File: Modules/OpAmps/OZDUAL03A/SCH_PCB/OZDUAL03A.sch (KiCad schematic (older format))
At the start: 53 parts, among them J1 JUMP2_2x1, J2 POWER, J3 OPAMPA, J4 OPAMPB, J5 VREF/TRANSISTOR, M1 HOLE, M2 HOLE, M3 HOLE, M4 HOLE, U1 OZ, U2 MAX6066

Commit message: uprava popisku
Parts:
- C1, C2, C3, C4: footprint Mlab_C:TantalC_SizeC_Reflow -> sot23-6:TantalC_SizeC_Reflow
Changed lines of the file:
@@
 F 0 "C1" H 6700 1350 50  0000 L CNN
 F 1 "47u" H 6700 1150 50  0000 L CNN
-F 2 "Mlab_C:TantalC_SizeC_Reflow" H 6700 1250 60  0001 C CNN
+F 2 "sot23-6:TantalC_SizeC_Reflow" H 6700 1250 60  0001 C CNN
 F 3 "" H 6700 1250 60  0000 C CNN
 	1    6700 1250
@@
 F 0 "C3" H 7400 1350 50  0000 L CNN
 F 1 "47u" H 7400 1150 50  0000 L CNN
-F 2 "Mlab_C:TantalC_SizeC_Reflow" H 7400 1250 60  0001 C CNN
+F 2 "sot23-6:TantalC_SizeC_Reflow" H 7400 1250 60  0001 C CNN
 F 3 "" H 7400 1250 60  0000 C CNN
 	1    7400 1250
@@
 F 0 "C2" H 6700 2050 50  0000 L CNN
 F 1 "47u" H 6700 1850 50  0000 L CNN
-F 2 "Mlab_C:TantalC_SizeC_Reflow" H 6700 1950 60  0001 C CNN
+F 2 "sot23-6:TantalC_SizeC_Reflow" H 6700 1950 60  0001 C CNN
 F 3 "" H 6700 1950 60  0000 C CNN
 	1    6700 1950
@@
 F 0 "C4" H 7400 2050 50  0000 L CNN
 F 1 "47u" H 7400 1850 50  0000 L CNN
-F 2 "Mlab_C:TantalC_SizeC_Reflow" H 7400 1950 60  0001 C CNN
+F 2 "sot23-6:TantalC_SizeC_Reflow" H 7400 1950 60  0001 C CNN
 F 3 "" H 7400 1950 60  0000 C CNN
 	1    7400 1950

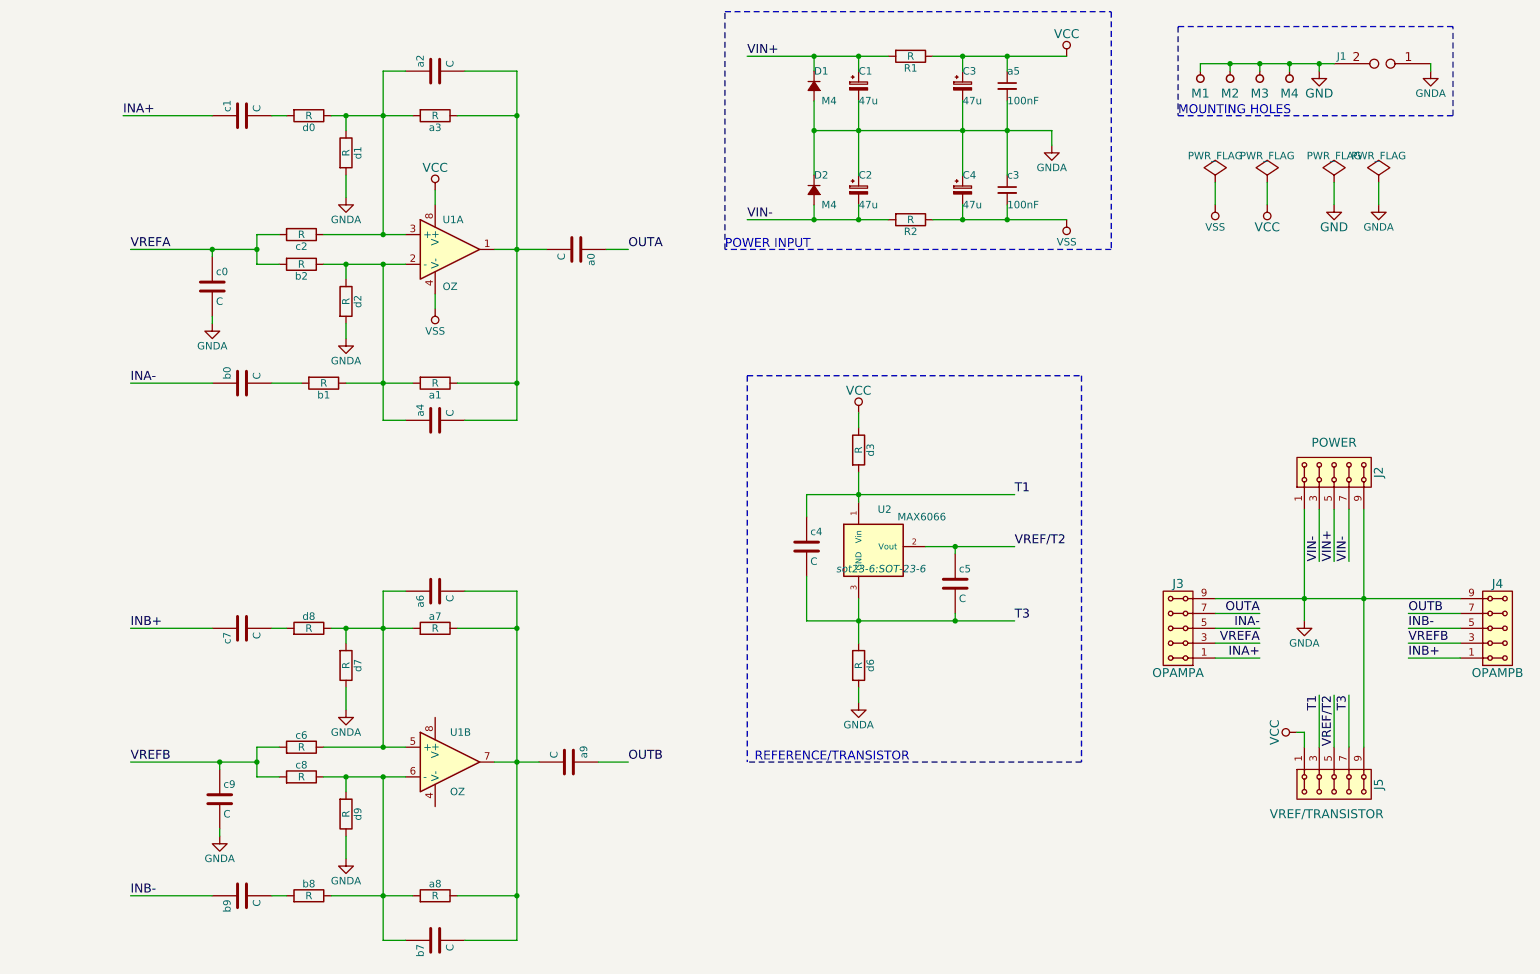
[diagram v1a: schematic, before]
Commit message: dalsi
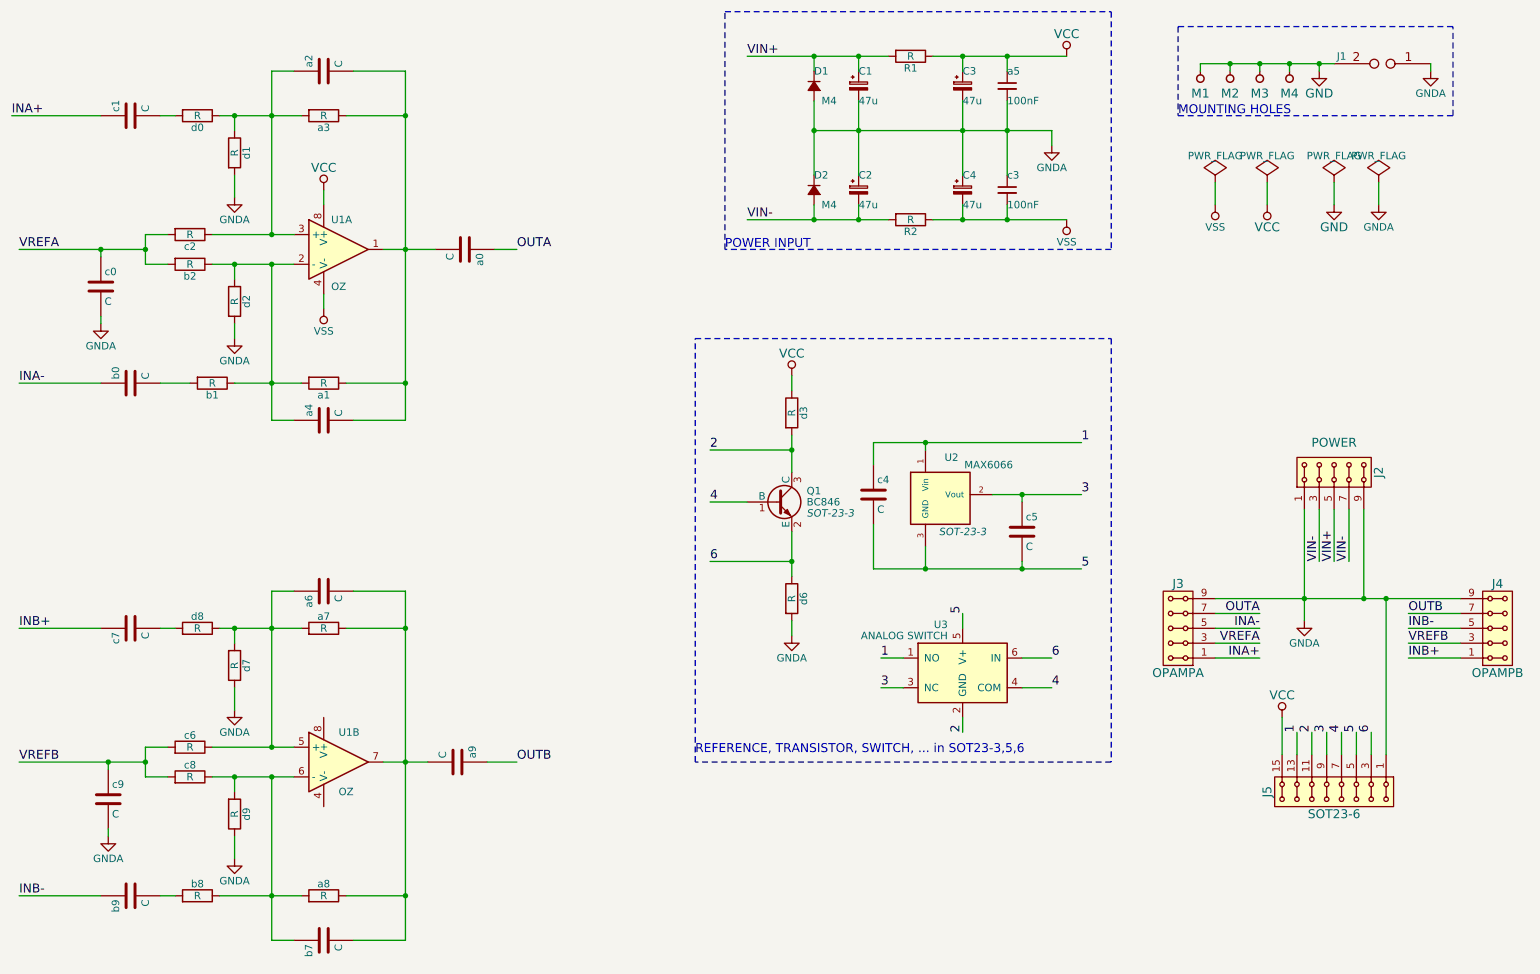
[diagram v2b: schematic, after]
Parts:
- removed J5: VREF/TRANSISTOR, Mlab_Pin_Headers:Straight_2x05, symbol HEADER_2x05_PARALLEL
- added J5: SOT23-6, Mlab_Pin_Headers:Straight_2x08, symbol HEADER_2x08_PARALLEL
- added Q1: BC846, SOT-23-3, symbol BC849
- added U3: ANALOG SWITCH, Mlab_IO:SOT-23-6, symbol TS5A3159
- U2: footprint sot23-6:SOT-23-6 -> SOT-23-3
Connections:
- net GNDA: now also J5.1, J5.2
- net VCC: now also J5.15, J5.16
- net T1 renamed 1
- net 1: now also J5.13, J5.14, U3.1 (NO); no longer d3.2
- net T3 renamed 5
- net 5: now also J5.5, J5.6, U3.5 (V+); no longer d6.1
- net VREF/T2 renamed 3
- net 3: now also J5.10, J5.9, U3.3 (NC)
- new net 2: J5.11, J5.12, Q1.3 (C), U3.2 (GND), d3.2
- new net 4: J5.7, J5.8, Q1.1 (B), U3.4 (COM)
- new net 6: J5.3, J5.4, Q1.2 (E), U3.6 (IN), d6.1
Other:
- note added: "REFERENCE, TRANSISTOR, SWITCH, ... in SOT23-3,5,6"
- note removed: "REFERENCE/TRANSISTOR"
- moved on the sheet: U1A, U1B, U2, a0, a1, a2, a3, a4, a6, a7, a8, a9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
